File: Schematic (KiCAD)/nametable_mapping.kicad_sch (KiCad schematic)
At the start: 40 parts

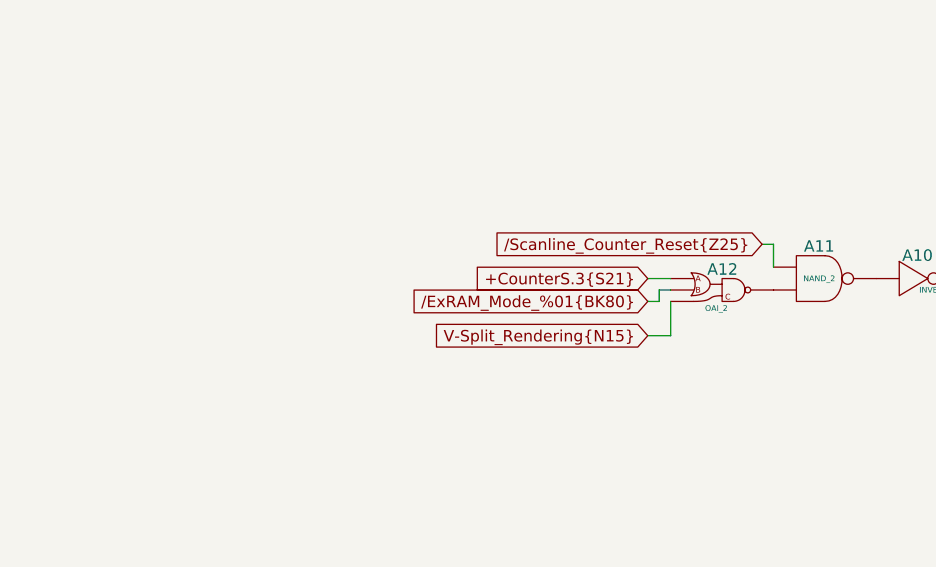
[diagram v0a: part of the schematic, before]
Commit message: Schematic and SVG Updates
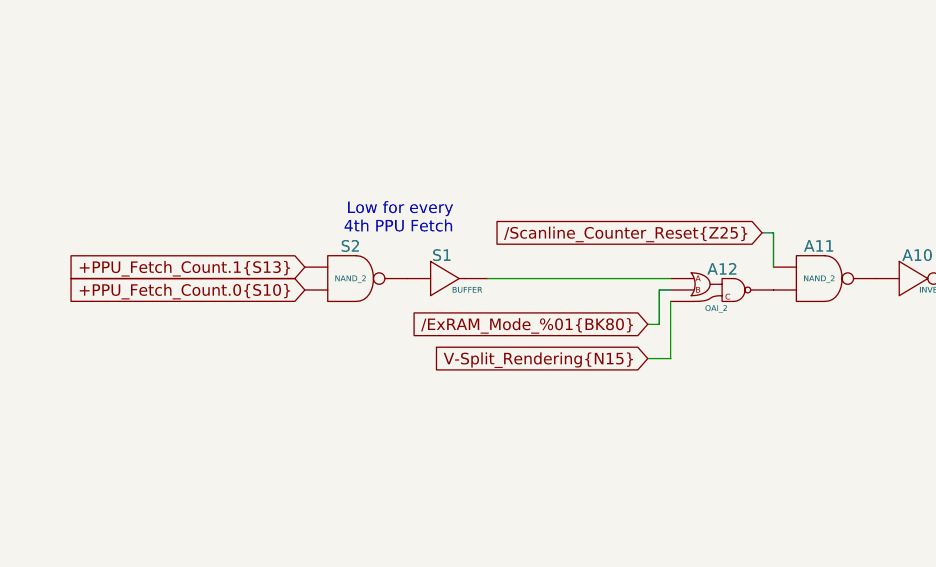
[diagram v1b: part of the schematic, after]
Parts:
- added S1: BUFFER, symbol MMC5:BUFFER
- added S2: NAND_2, symbol MMC5:NAND_2
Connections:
- net +CounterS.3{S21} is gone; now on net /ExRAM_Mode_%01{BK80}: A12. (X)
- new net: B9. (X), C1. (/Q7)
- new net: A13. (X), A14. (X), B18. (X), B19. (X), B20. (X), B21. (X), B22. (X), B23. (X), B24. (X), B25. (X)
- new net: A9. (Y4), B25. (X)
- new net: B6. (X), C1. (/Q7)
- new net: A9. (Y4), B23. (X)
- new net: A16. (X), B14. (X), B15. (X), B16. (X), B17. (X)
- new net: A13. (X), B14. (X), B15. (X), B16. (X), B17. (X)
- new net: A9. (Y4), B16. (X)
- new net: S1. (X), S2. (X)
- new net: B10. (X), C1. (/Q7)
- new net: A9. (Y4), B15. (X)
- new net: B7. (X), C1. (/Q7)
- new net: A11. (X), A12. (X)
- new net: A10. (X), A11. (X)
- new net: B4. (X), C1. (/Q7)
- new net: BL11. (X), BL33. (X)
- new net: B11. (X), C1. (/Q7)
- new net: A12. (X), S1. (X)
- new net: B3. (X), C1. (/Q7)
- new net: A9. (Y4), B22. (X)
- new net: A17. (X), C1. (/Q7)
- new net: A9. (Y4), B14. (X)
- new net: A9. (Y4), B21. (X)
- new net: A9. (Y4), B18. (X)
- new net: A9. (Y4), B20. (X)
- new net: A9. (Y4), B19. (X)
- new net: A9. (Y4), B17. (X)
- new net: A9. (Y4), B24. (X)
- new net: B13. (X), C1. (/Q7)
- new net: B12. (X), C1. (/Q7)
- new net: B5. (X), C1. (/Q7)
- new net: B8. (X), C1. (/Q7)
- new net +PPU_Fetch_Count.0{S10}: S2. (X)
- new net +PPU_Fetch_Count.1{S13}: S2. (X)
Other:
- note added: "Low for every 4th PPU Fetch"
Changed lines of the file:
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@@
 		)
 	)
+	(text "Low for every\n4th PPU Fetch"
+		(exclude_from_sim no)
+		(at 90.17 58.166 0)
+		(effects
+			(font
+				(size 1.27 1.27)
+			)
+			(justify right)
+		)
+	)
 	(text "Note: There is probably\nan inverter at each \noutput pin."
 		(exclude_from_sim no)
@@
 	(wire
 		(pts
-			(xy 111.76 67.31) (xy 113.03 67.31)
+			(xy 111.76 69.85) (xy 113.03 69.85)
 		)
 		(stroke
@@
 	(wire
 		(pts
-			(xy 111.76 64.77) (xy 114.3 64.77)
+			(xy 87.63 143.51) (xy 80.01 143.51)
 		)
 		(stroke
@@
 	(wire
 		(pts
-			(xy 87.63 143.51) (xy 80.01 143.51)
+			(xy 163.83 76.2) (xy 163.83 85.09)
 		)
 		(stroke
@@
 	(wire
 		(pts
-			(xy 163.83 76.2) (xy 163.83 85.09)
+			(xy 165.1 166.37) (xy 165.1 175.26)
 		)
 		(stroke
@@
 	(wire
 		(pts
-			(xy 165.1 166.37) (xy 165.1 175.26)
+			(xy 223.52 114.3) (xy 196.85 114.3)
 		)
 		(stroke
@@
 	(wire
 		(pts
-			(xy 223.52 114.3) (xy 196.85 114.3)
+			(xy 195.58 116.84) (xy 223.52 116.84)
 		)
 		(stroke
@@
 	(wire
 		(pts
-			(xy 195.58 116.84) (xy 223.52 116.84)
+			(xy 165.1 157.48) (xy 184.15 157.48)
 		)
 		(stroke
@@
 	(wire
 		(pts
-			(xy 165.1 157.48) (xy 184.15 157.48)
+			(xy 93.98 64.77) (xy 114.3 64.77)
 		)
 		(stroke
@@
 	(wire
 		(pts
-			(xy 125.73 60.96) (xy 125.73 63.5)
+			(xy 125.73 59.69) (xy 125.73 63.5)
 		)
 		(stroke
@@
 	(wire
 		(pts
-			(xy 111.76 71.12) (xy 114.3 71.12)
+			(xy 111.76 73.66) (xy 114.3 73.66)
 		)
 		(stroke
@@
 	(wire
 		(pts
-			(xy 113.03 66.04) (xy 113.03 67.31)
+			(xy 113.03 66.04) (xy 113.03 69.85)
 		)
 		(stroke
@@
 	(wire
 		(pts
-			(xy 114.3 71.12) (xy 114.3 67.31)
+			(xy 114.3 73.66) (xy 114.3 67.31)
 		)
 		(stroke
@@
 	(wire
 		(pts
-			(xy 124.46 60.96) (xy 125.73 60.96)
+			(xy 124.46 59.69) (xy 125.73 59.69)
 		)
 		(stroke
@@
 	(global_label "{slash}Scanline_Counter_Reset{Z25}"
 		(shape input)
-		(at 124.46 60.96 180)
+		(at 124.46 59.69 180)
 		(fields_autoplaced yes)
 		(effects
@@
 		)
 		(property "Intersheetrefs" "${INTERSHEET_REFS}"
-			(at 92.265 60.96 0)
+			(at 92.265 59.69 0)
 			(effects
 				(font
@@
 		)
 	)
-	(global_label "+CounterS.3{S21}"
-		(shape input)
-		(at 111.76 64.77 180)
-		(fields_autoplaced yes)
-		(effects
-			(font
-				(size 1.27 1.27)
-			)
-			(justify right)
-		)
-		(property "Intersheetrefs" "${INTERSHEET_REFS}"
-			(at 91.5392 64.77 0)
-			(effects
-				(font
-					(size 1.27 1.27)
-				)
-				(justify right)
-				(hide yes)
-			)
-		)
-	)
 	(global_label "+$5105.0{B3}"
 		(shape output)
@@
 		)
 	)
+	(global_label "+PPU_Fetch_Count.0{S10}"
+		(shape input)
+		(at 73.66 66.04 180)
+		(fields_autoplaced yes)
+		(effects
+			(font
+				(size 1.27 1.27)
+			)
+			(justify right)
+		)
+		(property "Intersheetrefs" "${INTERSHEET_REFS}"
+			(at 45.5773 66.04 0)
+			(effects
+				(font
+					(size 1.27 1.27)
+				)
+				(justify right)
+				(hide yes)
+			)
+		)
+	)
 	(global_label "CIRAM_CE_PIN{A9}"
 		(shape output)
@@
 	(global_label "V-Split_Rendering{N15}"
 		(shape input)
-		(at 111.76 71.12 180)
+		(at 111.76 73.66 180)
 		(fields_autoplaced yes)
 		(effects
@@
 		)
 		(property "Intersheetrefs" "${INTERSHEET_REFS}"
-			(at 85.9149 71.12 0)
+			(at 85.9149 73.66 0)
 			(effects
 				(font
@@
 		)
 	)
+	(global_label "+PPU_Fetch_Count.1{S13}"
+		(shape input)
+		(at 73.66 63.5 180)
+		(fields_autoplaced yes)
+		(effects
+			(font
+				(size 1.27 1.27)
+			)
+			(justify right)
+		)
+		(property "Intersheetrefs" "${INTERSHEET_REFS}"
+			(at 45.5773 63.5 0)
+			(effects
+				(font
+					(size 1.27 1.27)
+				)
+				(justify right)
+				(hide yes)
+			)
+		)
+	)
 	(global_label "+$5105.6{A17}"
 		(shape output)
@@
 	(global_label "{slash}ExRAM_Mode_%01{BK80}"
 		(shape input)
-		(at 111.76 67.31 180)
+		(at 111.76 69.85 180)
 		(fields_autoplaced yes)
 		(effects
@@
 		)
 		(property "Intersheetrefs" "${INTERSHEET_REFS}"
-			(at 84.1612 67.31 0)
+			(at 84.1612 69.85 0)
 			(effects
 				(font
@@
 	)
 	(symbol
+		(lib_name "NAND_2_45")
+		(lib_id "MMC5:NAND_2")
+		(at 78.74 64.77 0)
+		(unit 1)
+		(exclude_from_sim no)
+		(in_bom yes)
+		(on_board yes)
+		(dnp no)
+		(fields_autoplaced yes)
+		(property "Reference" "S2"
+			(at 78.74 60.452 0)
+			(do_not_autoplace yes)
+			(effects
+				(font
+					(size 1.27 1.27)
+				)
+				(justify top)
+			)
+		)
+		(property "Value" "NAND_2"
+			(at 78.74 64.77 0)
+			(do_not_autoplace yes)
+			(effects
+				(font
+					(size 0.635 0.635)
+				)
+			)
+		)
+		(property "Footprint" ""
+			(at 78.74 64.77 0)
+			(effects
+				(font
+					(size 1.27 1.27)
+				)
+				(hide yes)
+			)
+		)
+		(property "Datasheet" ""
+			(at 78.74 64.77 0)
+			(effects
+				(font
+					(size 1.27 1.27)
+				)
+				(hide yes)
+			)
+		)
+		(property "Description" ""
+			(at 78.74 64.77 0)
+			(effects
+				(font
+					(size 1.27 1.27)
+				)
+				(hide yes)
+			)
+		)
+		(pin ""
+		)
+		(pin ""
+		)
+		(pin ""
+		)
+		(instances
+			(project "MMC5"
+				(path "/46093bf6-f83e-4237-9ece-7350a682aff0/d931b895-16b8-4266-a6e9-dc595d1a00c0"
+					(reference "S2")
+					(unit 1)
+				)
+			)
+		)
+	)
+	(symbol
 		(lib_name "NAND_2_3")
 		(lib_id "MMC5:NAND_2")
@@
 					(unit 1)
 				)
+			)
+		)
+	)
+	(symbol
+		(lib_name "BUFFER_29")
+		(lib_id "MMC5:BUFFER")
+		(at 88.9 64.77 0)
+		(unit 1)
+		(exclude_from_sim no)
+		(in_bom yes)
+		(on_board yes)
+		(dnp no)
+		(fields_autoplaced yes)
+		(property "Reference" "S1"
+			(at 88.9 61.468 0)
+			(do_not_autoplace yes)
+			(effects
+				(font
+					(size 1.27 1.27)
+				)
+				(justify top)
+			)
+		)
+		(property "Value" "BUFFER"
+			(at 91.694 66.04 0)
+			(do_not_autoplace yes)
+			(effects
+				(font
+					(size 0.635 0.635)
+				)
+			)
+		)
+		(property "Footprint" ""
+			(at 88.9 64.77 0)
+			(effects
+				(font
+					(size 1.27 1.27)
+				)
+				(hide yes)
+			)
+		)
+		(property "Datasheet" ""
+			(at 88.9 64.77 0)
+			(effects
+				(font
+					(size 1.27 1.27)
+				)
+				(hide yes)
+			)
+		)
+		(property "Description" ""
+			(at 88.9 64.77 0)
+			(effects
+				(font
+					(size 1.27 1.27)
+				)
+				(hide yes)
+			)
+		)
+		(pin ""
+		)
+		(pin ""
+		)
+		(instances
+			(project "MMC5"
+				(path "/46093bf6-f83e-4237-9ece-7350a682aff0/d931b895-16b8-4266-a6e9-dc595d1a00c0"
+					(reference "S1")
+					(unit 1)
+				)
